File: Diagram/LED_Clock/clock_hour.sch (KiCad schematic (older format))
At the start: 28 parts, among them U4 MCP23017-E_SP

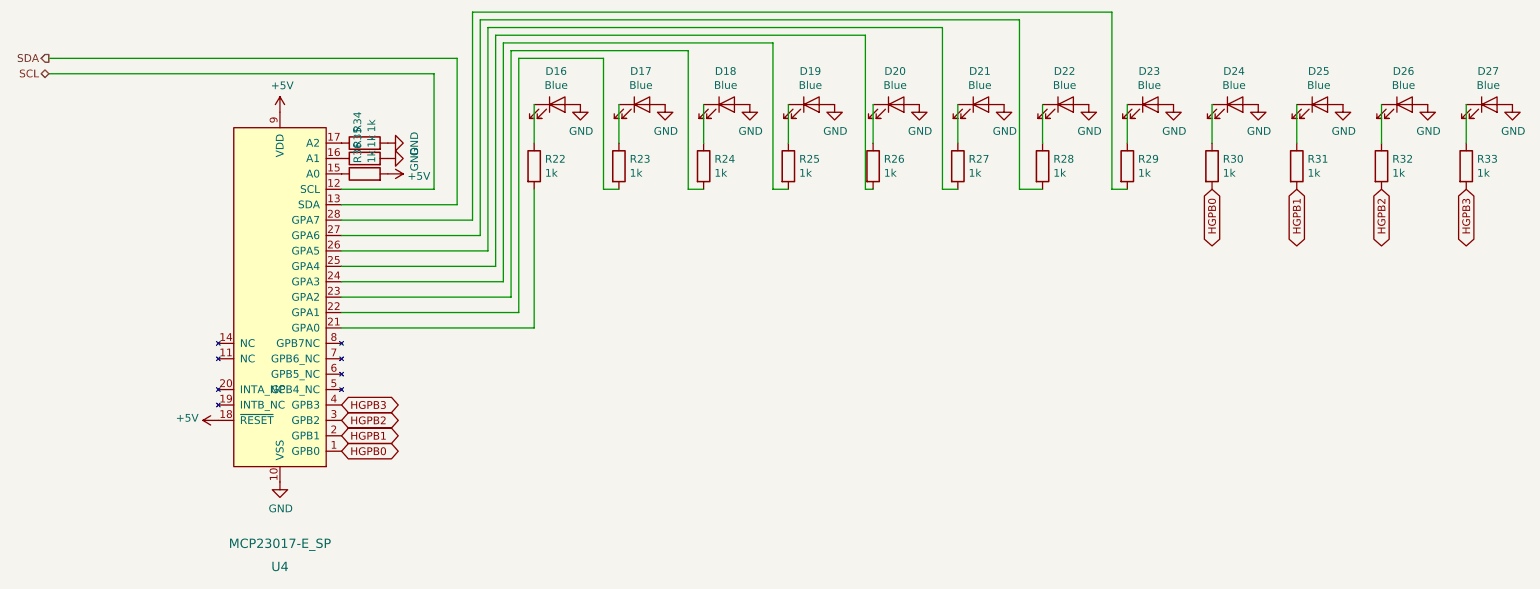
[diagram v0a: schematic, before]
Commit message: updated
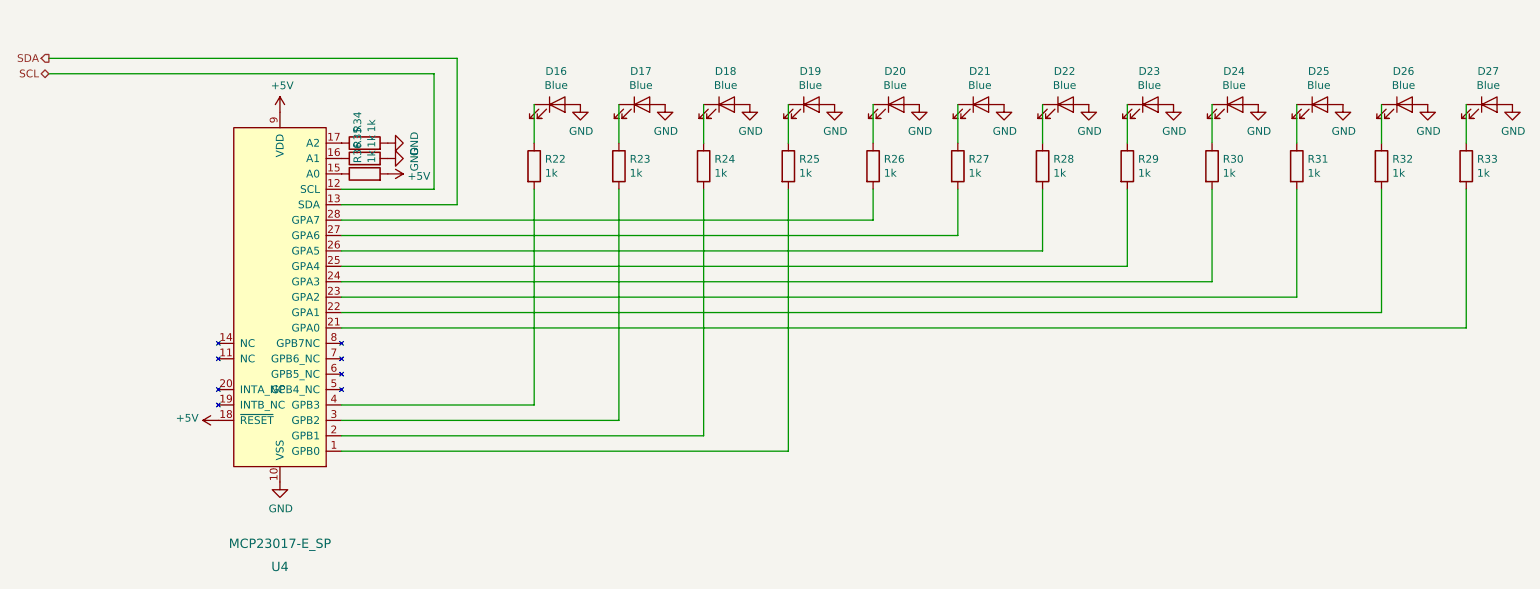
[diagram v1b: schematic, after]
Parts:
- renumbered U4 to U1
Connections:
- net at R22.2: now also U1.4 (GPB3); no longer U1.21 (GPA0)
- net at R25.2: now also U1.1 (GPB0); no longer U1.24 (GPA3)
- net at R26.2: now also U1.28 (GPA7); no longer U1.25 (GPA4)
- net at R27.2: now also U1.27 (GPA6); no longer U1.26 (GPA5)
- net at R28.2: now also U1.26 (GPA5); no longer U1.27 (GPA6)
- net at U1.22 (GPA1): now also R32.2; no longer R23.2
- net at U1.23 (GPA2): now also R31.2; no longer R24.2
- net at R29.2: now also U1.25 (GPA4); no longer U1.28 (GPA7)
- net HGPB0: no longer names the net of R30.2
- net HGPB0: now also U1.24 (GPA3); no longer U1.1 (GPB0)
- net HGPB1: no longer names the net of U1.2 (GPB1)
- net HGPB1: now also R24.2; no longer R31.2
- net HGPB2: no longer names the net of U1.3 (GPB2)
- net HGPB2: now also R23.2; no longer R32.2
- net HGPB3: no longer names the net of R33.2
- net HGPB3: now also U1.21 (GPA0); no longer U1.4 (GPB3)
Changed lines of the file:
@@
 $EndComp
 $Comp
-L LED_Clock-rescue:MCP23017-E_SP-dk_Interface-I-O-Expanders U?
+L LED_Clock-rescue:MCP23017-E_SP-dk_Interface-I-O-Expanders U1
 U 1 1 5E559BAD
 P 2400 3200
-AR Path="/5E559BAD" Ref="U?"  Part="1"
+AR Path="/5E559BAD" Ref="U1"  Part="1"
 AR Path="/5E4DDBDE/5E559BAD" Ref="U4"  Part="1"
 F 0 "U4" H 2500 4550 60  0000 C CNN
@@
 	-1   0    0    1
 $EndComp
-Wire Wire Line
-	2700 3000 3950 3000
-Wire Wire Line
-	3950 3000 3950 2100
-Wire Wire Line
-	2700 2900 3850 2900
-Wire Wire Line
-	3850 2900 3850 1250
-Wire Wire Line
-	3850 1250 4400 1250
-Wire Wire Line
-	4400 1250 4400 2100
-Wire Wire Line
-	4400 2100 4500 2100
-Wire Wire Line
-	2700 2800 3800 2800
-Wire Wire Line
-	3800 2800 3800 1200
-Wire Wire Line
-	3800 1200 4950 1200
-Wire Wire Line
-	4950 1200 4950 2100
-Wire Wire Line
-	4950 2100 5050 2100
-Wire Wire Line
-	2700 2700 3750 2700
-Wire Wire Line
-	3750 2700 3750 1150
-Wire Wire Line
-	3750 1150 5500 1150
-Wire Wire Line
-	5500 1150 5500 2100
-Wire Wire Line
-	5500 2100 5600 2100
-Wire Wire Line
-	2700 2600 3700 2600
-Wire Wire Line
-	3700 2600 3700 1100
-Wire Wire Line
-	3700 1100 6100 1100
-Wire Wire Line
-	6100 1100 6100 2100
-Wire Wire Line
-	6100 2100 6150 2100
-Wire Wire Line
-	3650 2500 3650 1050
-Wire Wire Line
-	3650 1050 6600 1050
-Wire Wire Line
-	6600 1050 6600 2100
-Wire Wire Line
-	6600 2100 6700 2100
-Wire Wire Line
-	2700 2500 3650 2500
-Wire Wire Line
-	2700 2400 3600 2400
-Wire Wire Line
-	3600 2400 3600 1000
-Wire Wire Line
-	3600 1000 7100 1000
-Wire Wire Line
-	7100 1000 7100 2100
-Wire Wire Line
-	7100 2100 7250 2100
-Wire Wire Line
-	2700 2300 3550 2300
-Wire Wire Line
-	3550 2300 3550 950
-Wire Wire Line
-	3550 950  7700 950
-Wire Wire Line
-	7700 950  7700 2100
-Wire Wire Line
-	7700 2100 7800 2100
-Text GLabel 8350 2100 3    50   BiDi ~ 0
-HGPB0
-Text GLabel 2700 3800 2    50   BiDi ~ 0
-HGPB0
-Text GLabel 2700 3700 2    50   BiDi ~ 0
-HGPB1
-Text GLabel 8900 2100 3    50   BiDi ~ 0
-HGPB1
-Text GLabel 9450 2100 3    50   BiDi ~ 0
-HGPB2
-Text GLabel 2700 3600 2    50   BiDi ~ 0
-HGPB2
-Text GLabel 2700 3500 2    50   BiDi ~ 0
-HGPB3
-Text GLabel 10000 2100 3    50   BiDi ~ 0
-HGPB3
 Text HLabel 800  1250 0    50   Output ~ 0
 SDA
@@
 AR Path="/5E4DDAEE/5E8FB0A2" Ref="#PWR?"  Part="1"
 AR Path="/5E4DDBDE/5E8FB0A2" Ref="#PWR0101"  Part="1"
+AR Path="/5E8FB0A2" Ref="#PWR0101"  Part="1"
 F 0 "#PWR0101" H 3000 1550 50  0001 C CNN
 F 1 "GND" H 3005 1627 50  0000 C CNN
@@
 AR Path="/5E4DDAEE/5E8FB0AE" Ref="#PWR?"  Part="1"
 AR Path="/5E4DDBDE/5E8FB0AE" Ref="#PWR0103"  Part="1"
+AR Path="/5E8FB0AE" Ref="#PWR0103"  Part="1"
 F 0 "#PWR0103" H 3000 1650 50  0001 C CNN
 F 1 "GND" H 3005 1727 50  0000 C CNN
@@
 AR Path="/5E4DDAEE/5E8FB0B4" Ref="R?"  Part="1"
 AR Path="/5E4DDBDE/5E8FB0B4" Ref="R34"  Part="1"
+AR Path="/5E8FB0B4" Ref="R34"  Part="1"
 F 0 "R34" H 2920 1846 50  0000 L CNN
 F 1 "1k" H 2920 1755 50  0000 L CNN
@@
 AR Path="/5E4DDAEE/5E8FB0BA" Ref="R?"  Part="1"
 AR Path="/5E4DDBDE/5E8FB0BA" Ref="R35"  Part="1"
+AR Path="/5E8FB0BA" Ref="R35"  Part="1"
 F 0 "R35" H 2920 1946 50  0000 L CNN
 F 1 "1k" H 2920 1855 50  0000 L CNN
@@
 AR Path="/5E4DDAEE/5E8FB0C0" Ref="R?"  Part="1"
 AR Path="/5E4DDBDE/5E8FB0C0" Ref="R36"  Part="1"
+AR Path="/5E8FB0C0" Ref="R36"  Part="1"
 F 0 "R36" H 2920 2046 50  0000 L CNN
 F 1 "1k" H 2920 1955 50  0000 L CNN
@@
 	0    1    1    0
 $EndComp
+Wire Wire Line
+	2700 3500 3950 3500
+Wire Wire Line
+	3950 3500 3950 2100
+Wire Wire Line
+	2700 3600 4500 3600
+Wire Wire Line
+	4500 3600 4500 2100
+Wire Wire Line
+	2700 3700 5050 3700
+Wire Wire Line
+	5050 3700 5050 2100
+Wire Wire Line
+	2700 3800 5600 3800
+Wire Wire Line
+	5600 3800 5600 2100
+Wire Wire Line
+	2700 2300 6150 2300
+Wire Wire Line
+	6150 2300 6150 2100
+Wire Wire Line
+	2700 2400 6700 2400
+Wire Wire Line
+	6700 2400 6700 2100
+Wire Wire Line
+	2700 2500 7250 2500
+Wire Wire Line
+	7250 2500 7250 2100
+Wire Wire Line
+	2700 2600 7800 2600
+Wire Wire Line
+	7800 2600 7800 2100
+Wire Wire Line
+	2700 2700 8350 2700
+Wire Wire Line
+	8350 2700 8350 2100
+Wire Wire Line
+	2700 2800 8900 2800
+Wire Wire Line
+	8900 2800 8900 2100
+Wire Wire Line
+	2700 2900 9450 2900
+Wire Wire Line
+	9450 2900 9450 2100
+Wire Wire Line
+	2700 3000 10000 3000
+Wire Wire Line
+	10000 3000 10000 2100
 $EndSCHEMATC
